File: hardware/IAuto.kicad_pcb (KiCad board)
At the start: 2 copper layers, 56 x 85 mm, 66 parts, among them J1 Barrel_Jack_Switch, J2 4R7uH, J3 4R7uH, J4 M1, J5 M2, J6 Cable_PAD, J7 Cable_PAD, J8 Cable_PAD, J9 Cable_PAD, P1 CONN_02X20, P2 CONN_02X05, Q1 SI4835DDY-T1-GE3, Q2 2N7002, Q3 2N7002, Q4 2N7002, Q5 2N7002, U1 ESP32_NODEMCU, U2 MP1584, U3 MP1584, U4 DRV8833

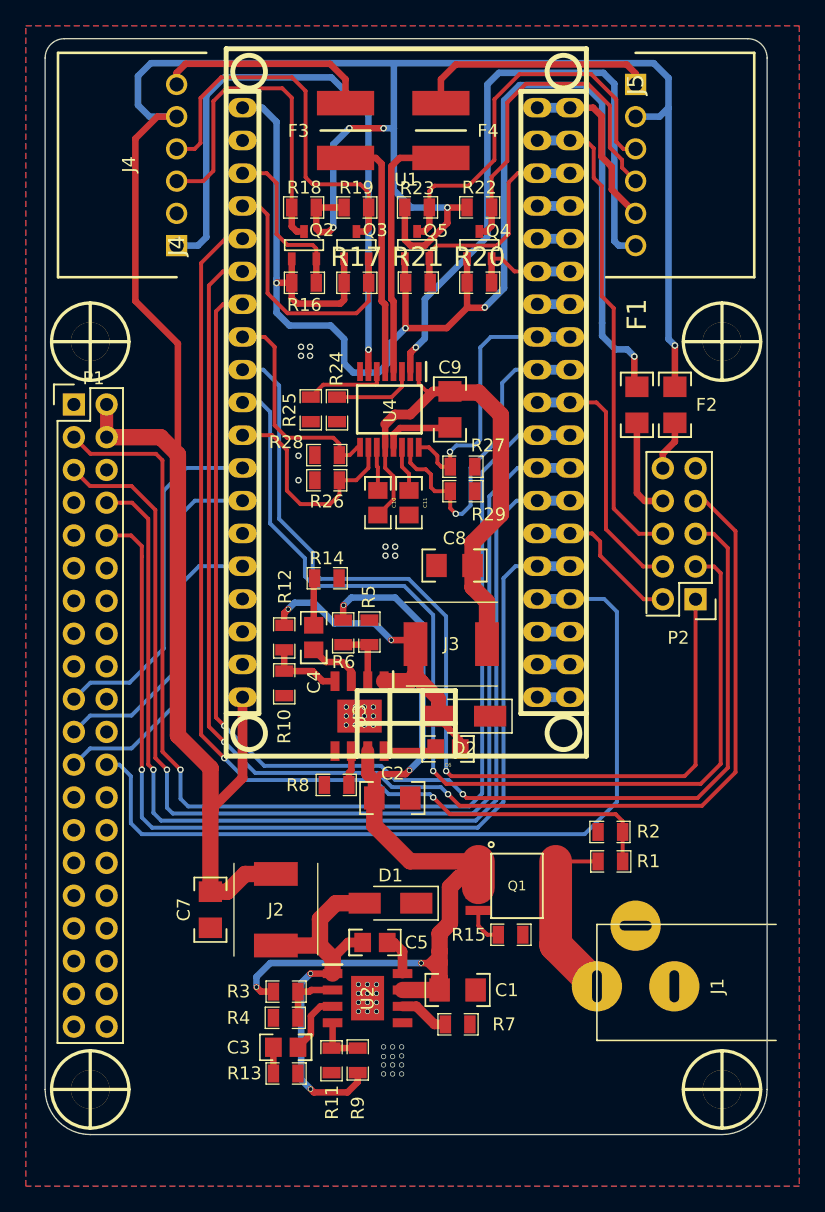
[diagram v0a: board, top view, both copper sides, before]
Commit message: Hardware
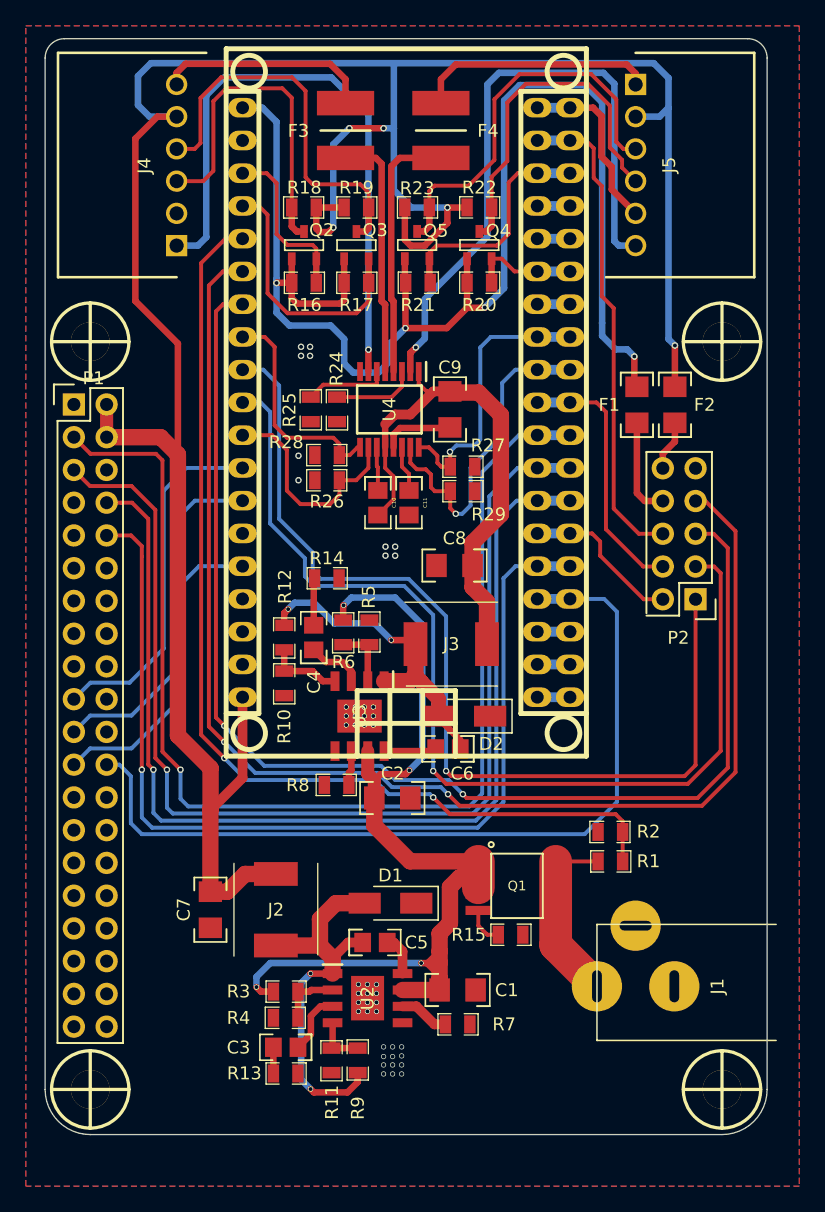
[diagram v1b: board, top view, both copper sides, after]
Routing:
- net /Logical Part/GPIO26: track 79.9 -> 79.3 mm
